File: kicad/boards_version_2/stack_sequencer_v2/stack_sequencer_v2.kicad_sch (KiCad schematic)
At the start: 10 parts

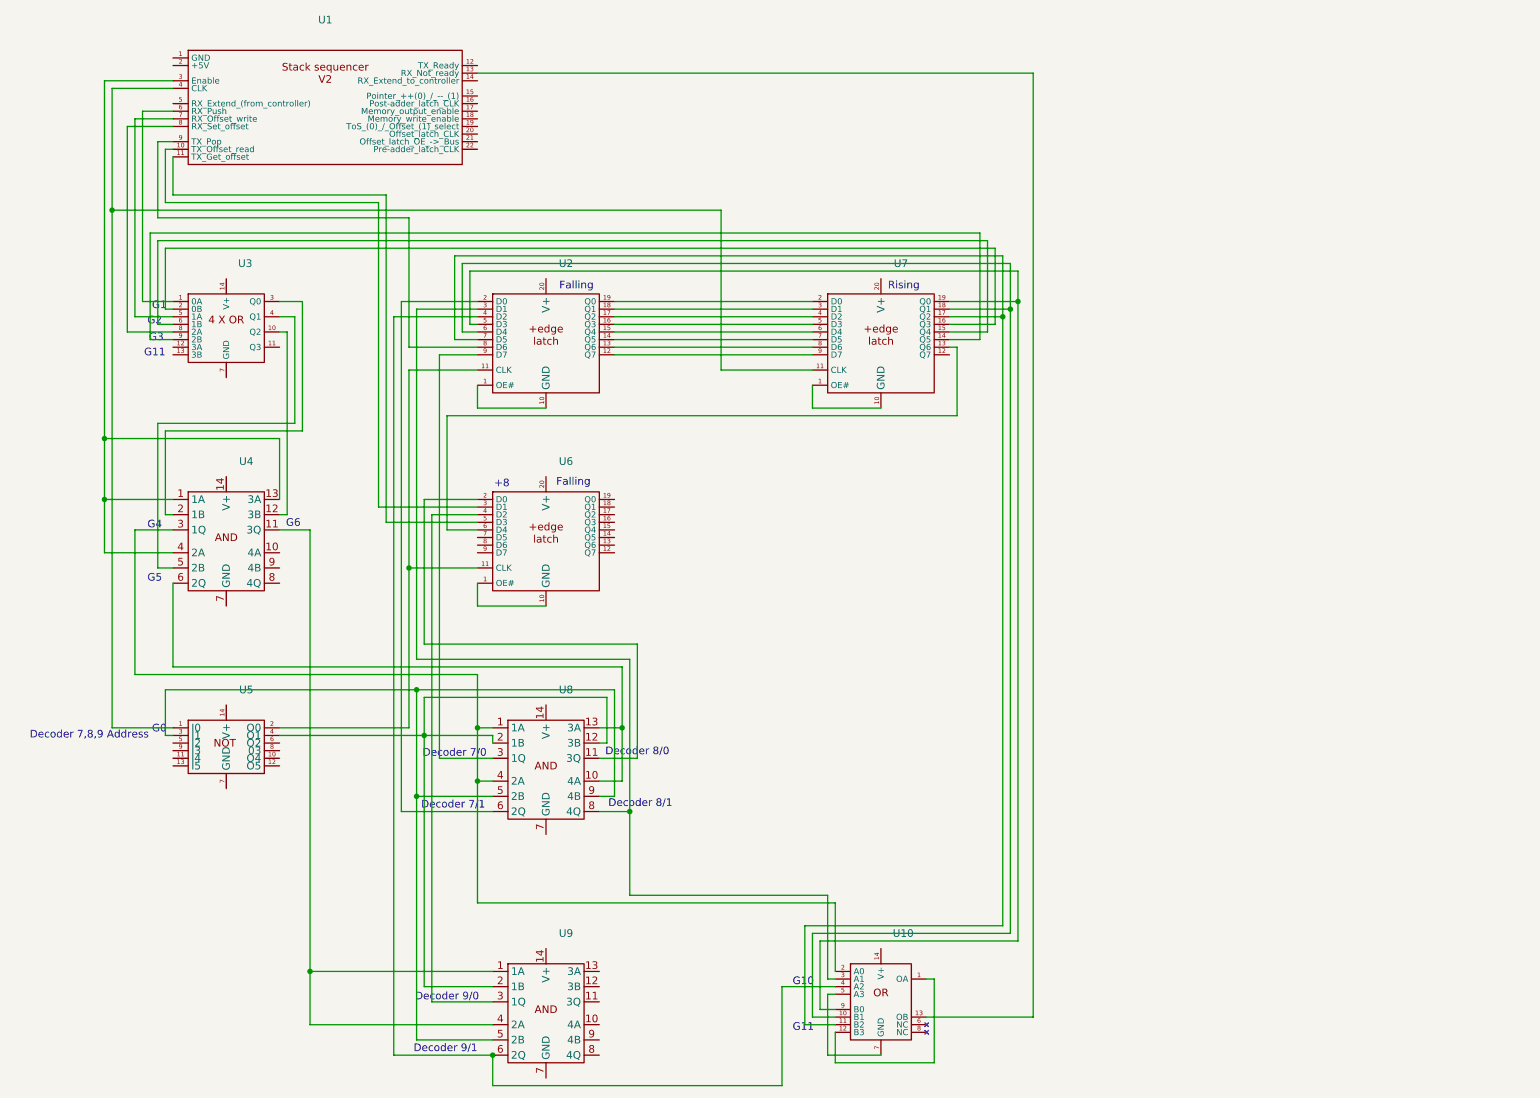
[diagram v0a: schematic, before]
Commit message: Work on stack sequencer
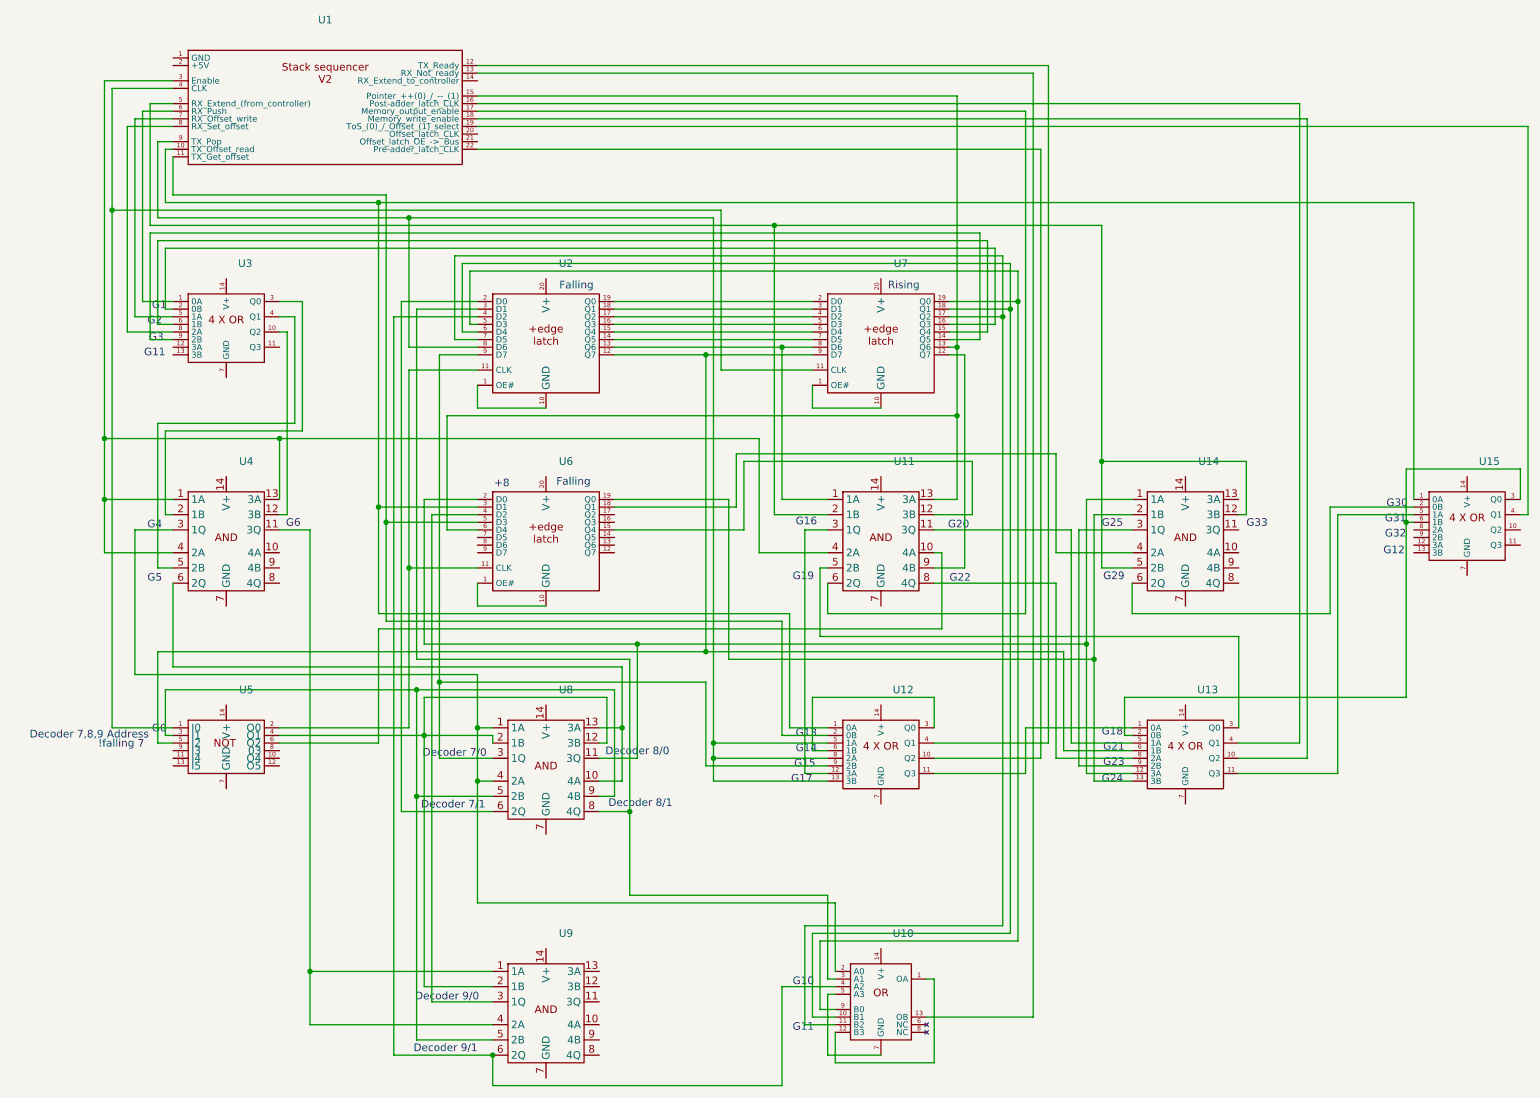
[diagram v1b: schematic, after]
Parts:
- added U11, U14: ~, Package_DIP:DIP-14_W7.62mm, symbol custom_symbol_lib:quad_and
- added U12, U13, U15: ~, Package_DIP:DIP-14_W7.62mm, symbol custom_symbol_lib:quad_OR
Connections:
- net at U7.12 (Q7): now also U11.9 (4B)
- net at U6.6 (D4), U7.13 (Q6): now also U1.15 (Pointer_++(0)_/_--_(1)), U11.13 (3A)
- net at U2.13 (Q6), U7.8 (D6): now also U11.1 (1A)
- net at U2.12 (Q7), U7.9 (D7): now also U5.5 (I2), U13.6 (1B)
- net at U6.15 (Q4): now also U11.12 (3B)
- net at U6.18 (Q1): now also U14.4 (2A)
- net at U6.19 (Q0): now also U13.13 (3B), U14.2 (1B)
- net at U6.2 (D0), U8.11 (3Q): now also U13.12 (3A), U14.1 (1A)
- net at U1.10 (TX_Offset_read), U6.3 (D1): now also U12.1 (0A), U15.1 (0A)
- net at U1.11 (TX_Get_offset), U6.5 (D3): now also U12.2 (0B)
- net at U1.3 (Enable), U4.1 (1A), U4.13 (3A)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: now also U11.4 (2A)
- net at U1.9 (TX_Pop), U2.8 (D6): now also U12.13 (3B), U12.5 (1A), U12.8 (2A)
- net at U2.9 (D7), U8.3 (1Q): now also U12.9 (2B)
- net at U5.6 (O2): now also U11.10 (4A)
- net at U1.12 (TX_Ready): now also U12.4 (Q1)
- net at U1.16 (Post-adder_latch_CLK): now also U13.4 (Q1)
- net at U1.17 (Memory_output_enable): now also U11.6 (2Q)
- net at U1.18 (Memory_write_enable): now also U13.10 (Q2)
- net at U1.19 (ToS_(0)_/_Offset_(1)_select): now also U15.4 (Q1)
- net at U1.22 (Pre-adder_latch_CLK): now also U12.10 (Q2)
- net at U1.5 (RX_Extend_(from_controller)): now also U11.2 (1B), U14.12 (3B), U14.5 (2B)
- new net: U12.11 (Q3), U13.1 (0A)
- new net: U13.11 (Q3), U15.5 (1A)
- new net: U13.2 (0B), U15.3 (Q0), U15.6 (1B)
- new net: U11.5 (2B), U13.3 (Q0)
- new net: U11.11 (3Q), U13.5 (1A)
- new net: U11.8 (4Q), U13.8 (2A)
- new net: U13.9 (2B), U14.3 (1Q)
- new net: U14.6 (2Q), U15.2 (0B)
- new net: U11.3 (1Q), U12.12 (3A)
- new net: U12.3 (Q0), U12.6 (1B)
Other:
- note added: "!falling 7"
- note added: "G12"
- note added: "G13"
- note added: "G14"
- note added: "G15"
- note added: "G16"
- note added: "G17"
- note added: "G18"
- note added: "G19"
- note added: "G20"
- note added: "G21"
- note added: "G22"
- note added: "G23"
- note added: "G24"
- note added: "G25"
- note added: "G29"
- note added: "G30"
- note added: "G31"
- note added: "G32"
- note added: "G33"
